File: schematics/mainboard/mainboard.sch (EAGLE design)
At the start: 75 parts, among them IC1 OPA2344P, IC2 74AHC00D, IC3 LM2576-5.0, IC4 LM2576-3.3, Q1 BD140, Q2 BD140, Q3 IRF540, U1 STM32F777VIT

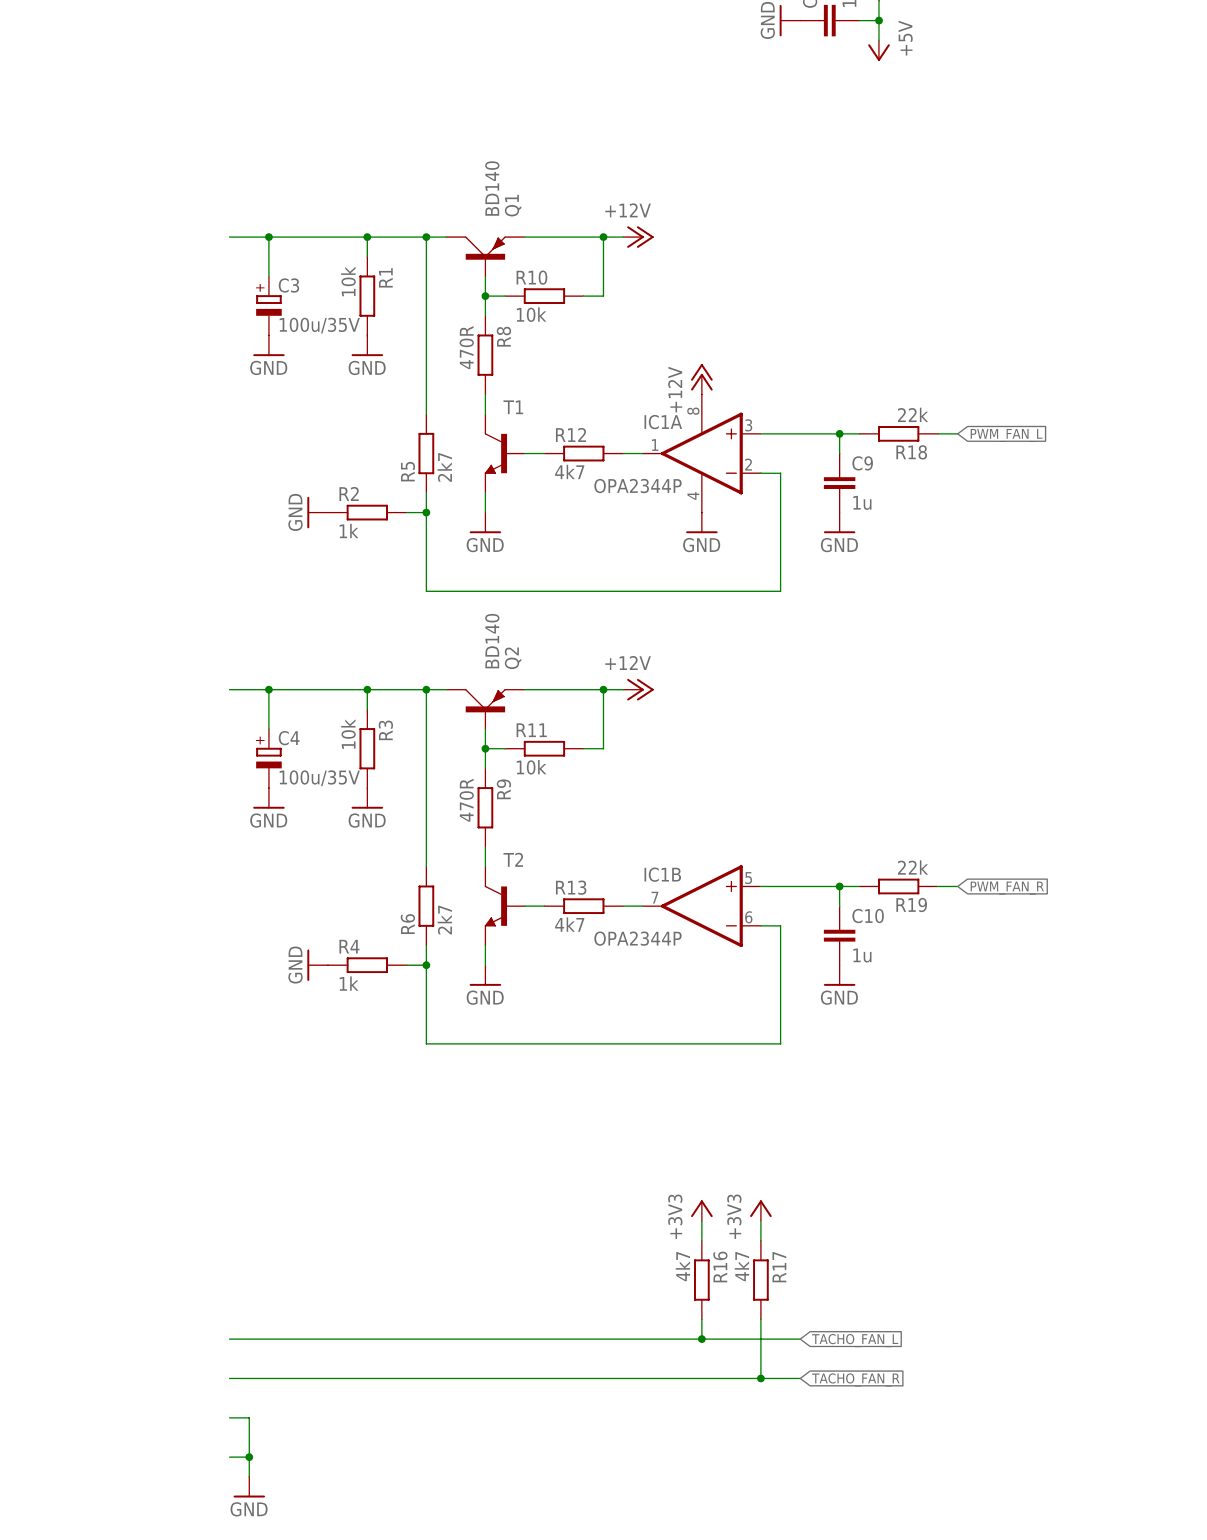
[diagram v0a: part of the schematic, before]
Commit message: Add files via upload
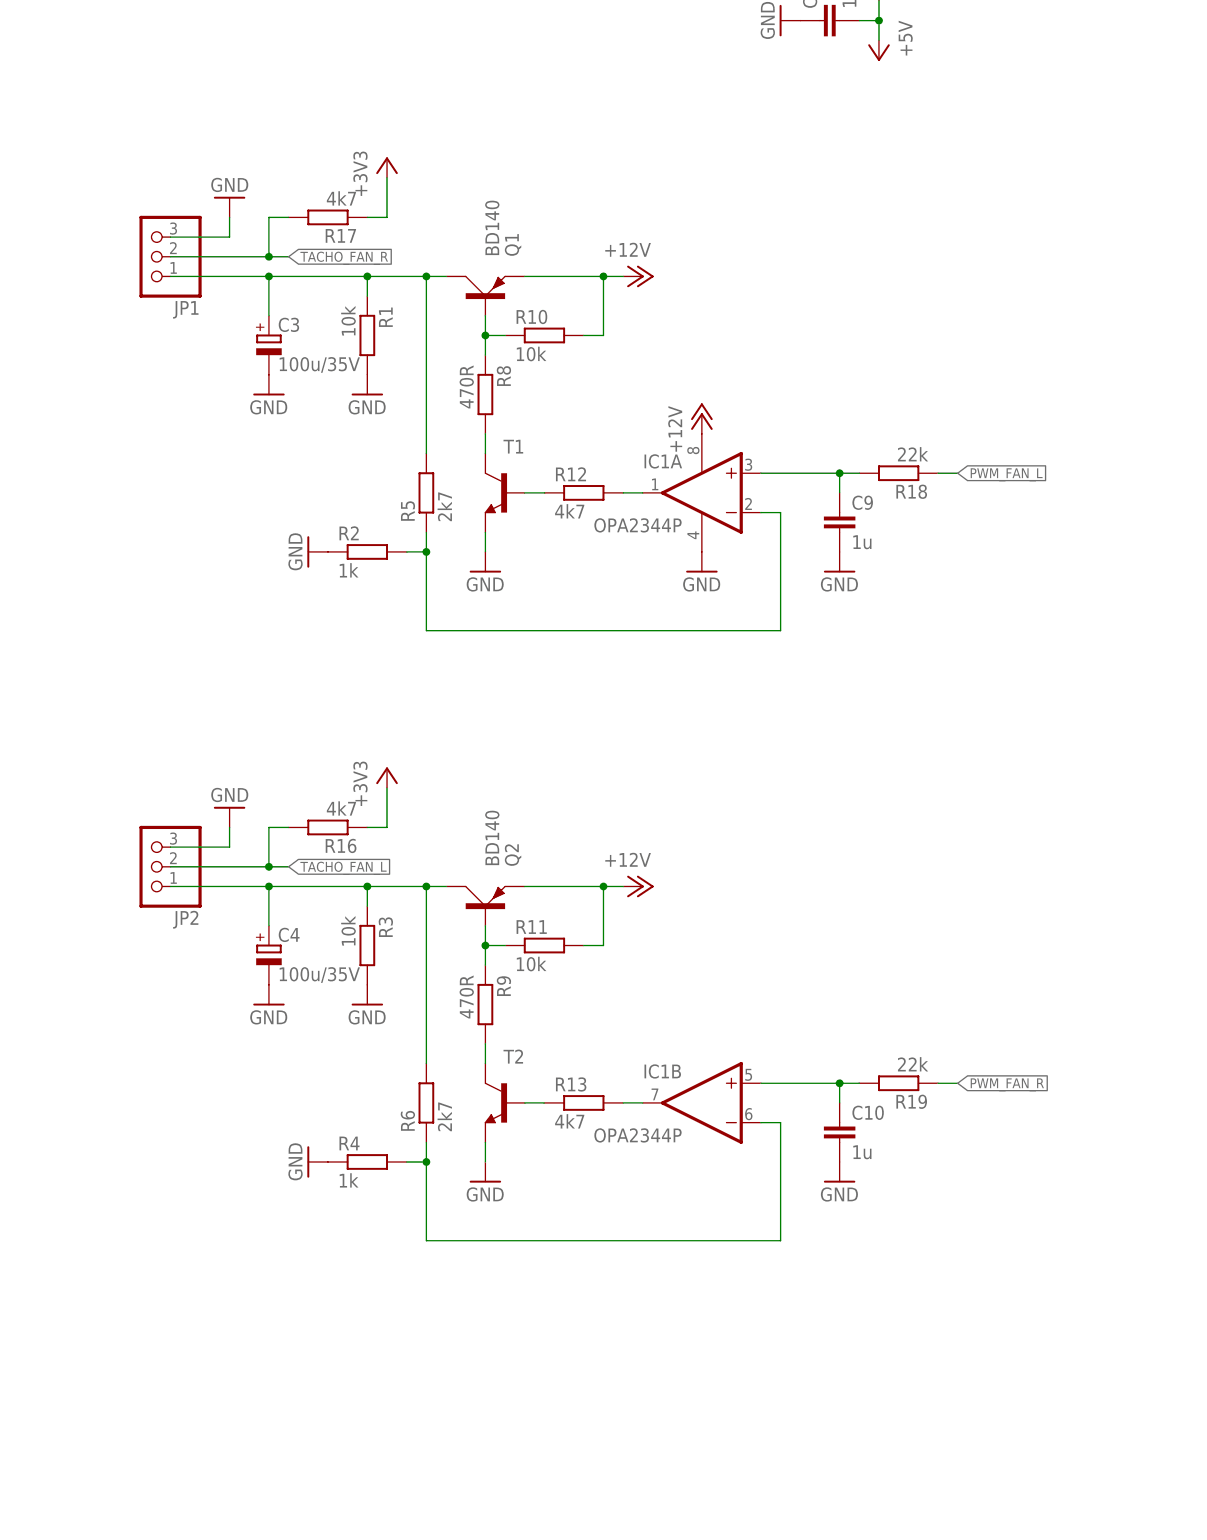
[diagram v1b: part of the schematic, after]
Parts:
- added JP1, JP2: (no value), pinhead:PINHD-1X3
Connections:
- net GND: now also JP1.3, JP2.3
- net N$15: now also JP1.1
- net N$19: now also JP2.1
- net TACHO_FAN_L: now also JP2.2
- net TACHO_FAN_R: now also JP1.2
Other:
- moved on the sheet: C10, C3, C4, C9, IC1A, IC1B, Q1, Q2, R1, R10, R11, R12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

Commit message: Add files via upload
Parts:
- added C26, C27: 22u/25, rcl:CPOL-EUE2-5
- added C28, C29: 100n, rcl:C-EUC0805
- added C30: 4.7u, rcl:C-EUC0805
- added IC5: LM339N, linear:LM339N
- added R20, R21, R25: 4k7, resistor:R-EU_R0805
- added R22: 2k7, resistor:R-EU_R0805
- added R23, R24: (no value), rcl:R-TRIMM3296W
- R17: value 4k7 -> 2k7
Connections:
- new net L_FAN_OK: IC5A.OUT, IC5B.OUT, R20.2
- new net N$26: C26.+, IC5C.+IN, IC5D.+IN, R16.1, R17.2
- new net N$27: C27.+, IC5A.-IN, IC5B.+IN, R21.1, R22.2
- new net R_FAN_OK: IC5C.OUT, IC5D.OUT, R25.2
- new net V_DN: C29.1, IC5B.-IN, IC5D.-IN, R23.S
- new net V_UP: C28.1, IC5A.+IN, IC5C.-IN, R24.S
- net +3V3: now also C30.1, IC5P.V+, R20.1, R22.1, R23.E, R24.E, R25.1; no longer R16.1
- net GND: now also C26.-, C27.-, C28.2, C29.2, C30.2, IC5P.GND, R23.A, R24.A
- net TACHO_FAN_L: now also R21.2; no longer R16.2
- net TACHO_FAN_R: now also R16.2; no longer R17.2
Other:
- moved on the sheet: R16, R17
